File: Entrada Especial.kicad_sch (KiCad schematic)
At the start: 57 parts, among them U30 TLV9301xDBV, U31 TLV9301xDBV, U32 LM7705, U33 MCP1799T-5002H/TT

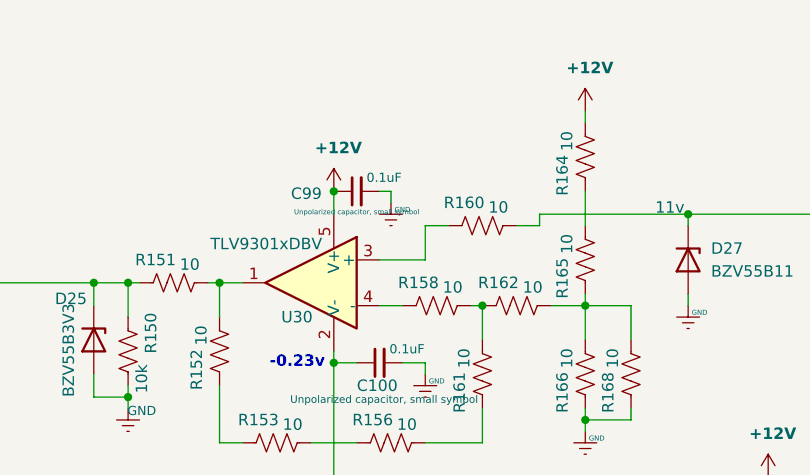
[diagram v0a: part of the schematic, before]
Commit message: 14-JUL-26
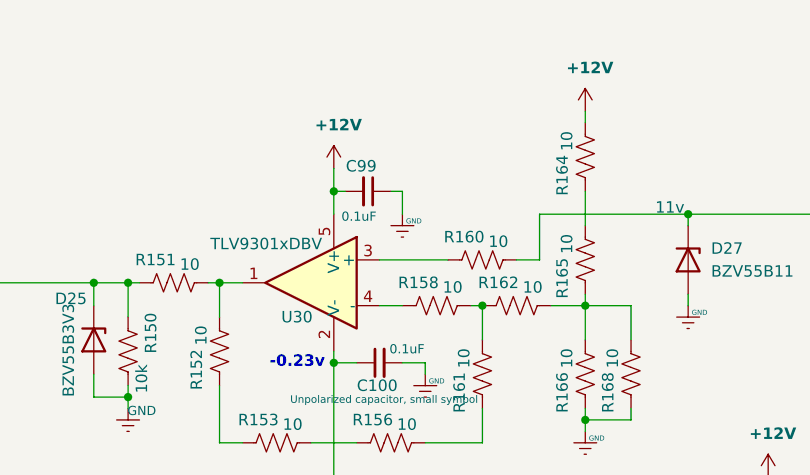
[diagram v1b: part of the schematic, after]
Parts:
- C99: now in the parts list
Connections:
- net +12V: now also C99.2; no longer C99.1
- net GND: now also C99.1; no longer C99.2
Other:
- moved on the sheet: R160
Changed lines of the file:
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@@
 	)
 	(junction
-		(at 77.47 67.31)
-		(diameter 0)
-		(color 0 0 0 0)
-	)
-	(junction
 		(at 77.47 86.36)
 		(diameter 0)
@@
 	)
 	(junction
+		(at 77.47 67.31)
+		(diameter 0)
+		(color 0 0 0 0)
+	)
+	(junction
 		(at 140.97 154.94)
 		(diameter 0)
@@
 	(wire
 		(pts
-			(xy 93.98 95.25) (xy 93.98 91.44)
+			(xy 77.47 67.31) (xy 77.47 69.85)
 		)
 		(stroke
@@
 	(wire
 		(pts
-			(xy 87.63 74.93) (xy 87.63 71.12)
+			(xy 93.98 95.25) (xy 93.98 91.44)
 		)
 		(stroke
@@
 	(wire
 		(pts
-			(xy 87.63 71.12) (xy 90.17 71.12)
-		)
-		(stroke
-			(width 0)
-			(type default)
-		)
-	)
-	(wire
-		(pts
 			(xy 243.84 102.87) (xy 251.46 102.87)
 		)
@@
 	(wire
 		(pts
-			(xy 82.55 67.31) (xy 83.82 67.31)
-		)
-		(stroke
-			(width 0)
-			(type default)
-		)
-	)
-	(wire
-		(pts
 			(xy 120.65 110.49) (xy 137.16 110.49)
 		)
@@
 	(wire
 		(pts
-			(xy 100.33 71.12) (xy 100.33 69.85)
+			(xy 100.33 74.93) (xy 100.33 69.85)
 		)
 		(stroke
@@
 	(wire
 		(pts
-			(xy 97.79 71.12) (xy 100.33 71.12)
+			(xy 97.79 74.93) (xy 100.33 74.93)
 		)
 		(stroke
@@
 	(wire
 		(pts
-			(xy 82.55 74.93) (xy 87.63 74.93)
+			(xy 82.55 74.93) (xy 90.17 74.93)
 		)
 		(stroke
@@
 	(wire
 		(pts
+			(xy 85.09 67.31) (xy 83.82 67.31)
+		)
+		(stroke
+			(width 0)
+			(type default)
+		)
+	)
+	(wire
+		(pts
 			(xy 110.49 92.71) (xy 105.41 92.71)
 		)
@@
 	(wire
 		(pts
+			(xy 78.74 67.31) (xy 77.47 67.31)
+		)
+		(stroke
+			(width 0)
+			(type default)
+		)
+	)
+	(wire
+		(pts
 			(xy 170.18 133.35) (xy 170.18 130.81)
 		)
@@
 	(wire
 		(pts
-			(xy 77.47 67.31) (xy 77.47 69.85)
+			(xy 77.47 64.77) (xy 77.47 67.31)
 		)
 		(stroke
@@
 	(wire
 		(pts
-			(xy 83.82 67.31) (xy 83.82 68.58)
+			(xy 85.09 67.31) (xy 85.09 69.85)
 		)
 		(stroke
@@
 	(symbol
 		(lib_id "power:+12V")
-		(at 77.47 67.31 0)
+		(at 77.47 64.77 0)
 		(mirror y)
 		(unit 1)
@@
 		(dnp no)
 		(property "Reference" "#PWR0364"
-			(at 77.47 71.12 0)
+			(at 77.47 68.58 0)
 			(effects
 				(font
@@
 		)
 		(property "Value" "+12V"
-			(at 77.978 62.484 0)
+			(at 77.978 59.944 0)
 			(effects
 				(font
@@
 		)
 		(property "Footprint" ""
-			(at 77.47 67.31 0)
+			(at 77.47 64.77 0)
 			(effects
 				(font
@@
 		)
 		(property "Datasheet" ""
-			(at 77.47 67.31 0)
+			(at 77.47 64.77 0)
 			(effects
 				(font
@@
 		)
 		(property "Description" "Power symbol creates a global label with name \"+12V\""
-			(at 77.47 67.31 0)
+			(at 77.47 64.77 0)
 			(effects
 				(font
@@
 	(symbol
 		(lib_id "Device:R_US")
-		(at 93.98 71.12 270)
+		(at 93.98 74.93 270)
 		(unit 1)
 		(exclude_from_sim no)
@@
 		(dnp no)
 		(property "Reference" "R160"
-			(at 91.948 68.58 90)
+			(at 91.948 72.39 90)
 			(effects
 				(font
@@
 		)
 		(property "Value" "10"
-			(at 95.758 69.088 90)
+			(at 95.758 72.898 90)
 			(effects
 				(font
@@
 		)
 		(property "Footprint" "Resistor_SMD:R_0603_1608Metric"
-			(at 93.726 72.136 90)
+			(at 93.726 75.946 90)
 			(effects
 				(font
@@
 		)
 		(property "Datasheet" "~"
-			(at 93.98 71.12 0)
+			(at 93.98 74.93 0)
 			(effects
 				(font
@@
 		)
 		(property "Description" "Resistor, US symbol"
-			(at 93.98 71.12 0)
+			(at 93.98 74.93 0)
 			(effects
 				(font
@@
 	(symbol
 		(lib_id "Device:C_Small")
+		(at 81.28 67.31 270)
+		(mirror x)
+		(unit 1)
+		(exclude_from_sim no)
+		(in_bom yes)
+		(on_board yes)
+		(dnp no)
+		(property "Reference" "C99"
+			(at 80.518 64.516 90)
+			(effects
+				(font
+					(size 1.27 1.27)
+				)
+			)
+		)
+		(property "Value" "0.1uF"
+			(at 80.264 70.104 90)
+			(effects
+				(font
+					(size 1.016 1.016)
+				)
+			)
+		)
+		(property "Footprint" "Capacitor_SMD:C_0603_1608Metric_Pad1.08x0.95mm_HandSolder"
+			(at 81.28 67.31 0)
+			(effects
+				(font
+					(size 1.27 1.27)
+				)
+				(hide yes)
+			)
+		)
+		(property "Datasheet" "~"
+			(at 81.28 67.31 0)
+			(effects
+				(font
+					(size 1.27 1.27)
+				)
+				(hide yes)
+			)
+		)
+		(property "Description" "Unpolarized capacitor, small symbol"
+			(at 81.28 67.31 0)
+			(effects
+				(font
+					(size 1.27 1.27)
+				)
+				(hide yes)
+			)
+		)
+		(pin "2"
+		)
+		(pin "1"
+		)
+		(instances
+			(project "01_IO-ASD-PLUS"
+				(path "/38a2da3c-ed29-422f-ab41-066ccf490e61/19faad97-cb14-41b6-a038-81c575645464"
+					(reference "C99")
+					(unit 1)
+				)
+			)
+		)
+	)
+	(symbol
+		(lib_id "Device:C_Small")
 		(at 204.47 135.89 0)
 		(mirror x)
@@
 	)
 	(symbol
-		(lib_id "Device:C_Small")
-		(at 80.01 67.31 90)
-		(unit 1)
-		(exclude_from_sim no)
-		(in_bom no)
-		(on_board no)
-		(dnp no)
-		(property "Reference" "C99"
-			(at 74.422 67.564 90)
-			(effects
-				(font
-					(size 1.27 1.27)
-				)
-			)
-		)
-		(property "Value" "0.1uF"
-			(at 83.058 65.786 90)
-			(effects
-				(font
-					(size 1.016 1.016)
-				)
-			)
-		)
-		(property "Footprint" "Capacitor_SMD:C_0603_1608Metric_Pad1.08x0.95mm_HandSolder"
-			(at 80.01 67.31 0)
-			(effects
-				(font
-					(size 1.27 1.27)
-				)
-				(hide yes)
-			)
-		)
-		(property "Datasheet" "~"
-			(at 80.01 67.31 0)
-			(effects
-				(font
-					(size 1.27 1.27)
-				)
-				(hide yes)
-			)
-		)
-		(property "Description" "Unpolarized capacitor, small symbol"
-			(at 80.01 69.596 90)
-			(effects
-				(font
-					(size 0.5588 0.5588)
-				)
-			)
-		)
-		(pin "2"
-		)
-		(pin "1"
-		)
-		(instances
-			(project "01_IO-ASD-PLUS"
-				(path "/38a2da3c-ed29-422f-ab41-066ccf490e61/19faad97-cb14-41b6-a038-81c575645464"
-					(reference "C99")
-					(unit 1)
-				)
-			)
-		)
-	)
-	(symbol
 		(lib_id "power:GNDREF")
 		(at 140.97 163.83 0)
@@
 	(symbol
 		(lib_id "power:GNDREF")
-		(at 83.82 68.58 0)
+		(at 85.09 69.85 0)
 		(unit 1)
 		(exclude_from_sim no)
@@
 		(dnp no)
 		(property "Reference" "#PWR0365"
-			(at 83.82 74.93 0)
+			(at 85.09 76.2 0)
 			(effects
 				(font
@@
 		)
 		(property "Value" "GND"
-			(at 85.09 69.342 0)
+			(at 86.36 70.612 0)
 			(effects
 				(font
@@
 		)
 		(property "Footprint" ""
-			(at 83.82 68.58 0)
+			(at 85.09 69.85 0)
 			(effects
 				(font
@@
 		)
 		(property "Datasheet" ""
-			(at 83.82 68.58 0)
+			(at 85.09 69.85 0)
 			(effects
 				(font
@@
 		)
 		(property "Description" "Power symbol creates a global label with name \"GNDREF\" , reference supply ground"
-			(at 83.82 68.58 0)
+			(at 85.09 69.85 0)
 			(effects
 				(font

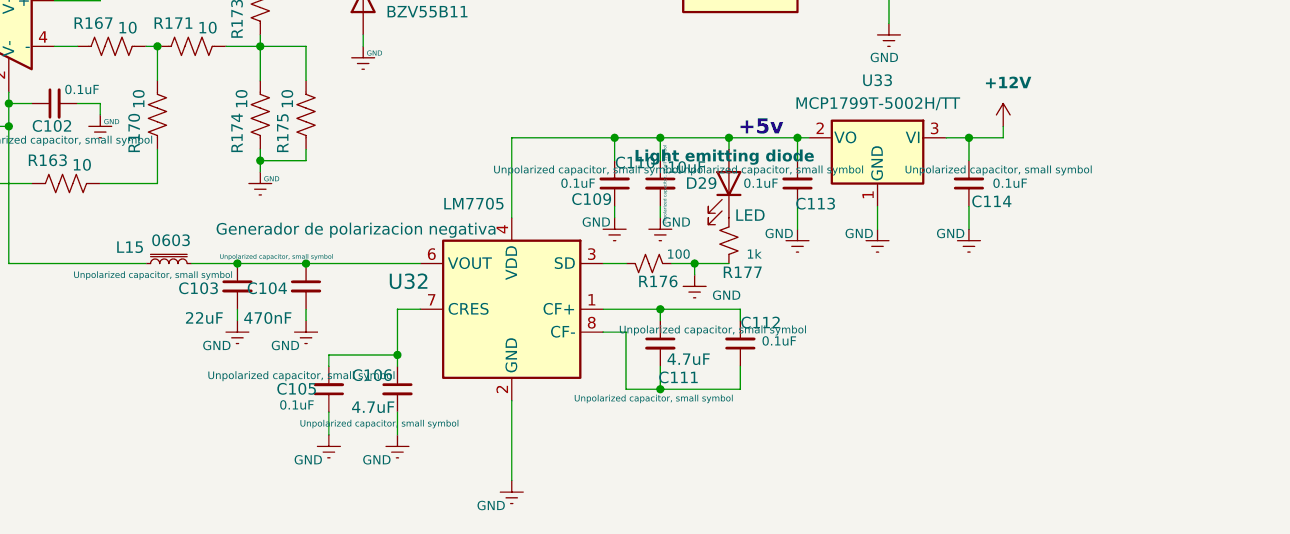
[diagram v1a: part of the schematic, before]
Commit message: 17-07-26
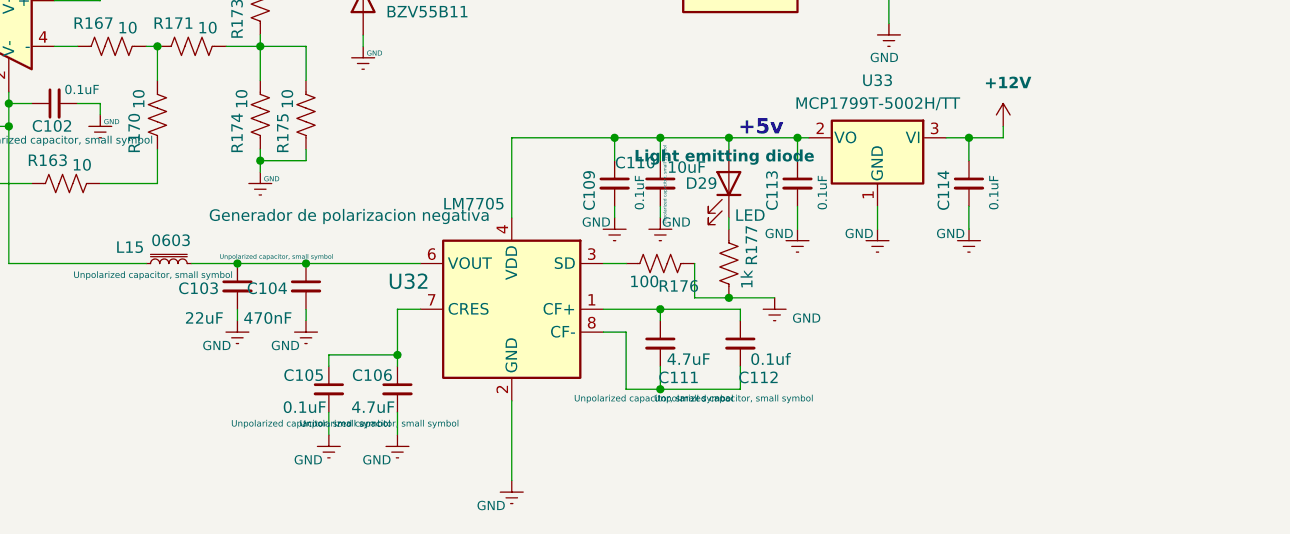
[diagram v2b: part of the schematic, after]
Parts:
- removed R176: 100, Resistor_SMD:R_0603_1608Metric_Pad0.98x0.95mm_HandSolder, symbol Device:R_Small_US
- removed R177: 1k, Resistor_SMD:R_0603_1608Metric_Pad0.98x0.95mm_HandSolder, symbol Device:R_Small_US
- added R176: 100, Resistor_SMD:R_0603_1608Metric, symbol Device:R_US
- added R177: 1k, Resistor_SMD:R_0603_1608Metric, symbol Device:R_US
- C105: footprint Capacitor_SMD:C_0603_1608Metric_Pad1.08x0.95mm_HandSolder -> Capacitor_SMD:C_0603_1608Metric; Mouser (none) -> 81-GCJ188M8EC475KE8D; Price (none) -> 0.416; now in the parts list
- C109, C113, C114: now in the parts list
- C112: value 0.1uF -> 0.1uf; footprint Capacitor_SMD:C_0603_1608Metric_Pad1.08x0.95mm_HandSolder -> Capacitor_SMD:C_0603_1608Metric; Mouser (none) -> 81-GCJ188M8EC475KE8D; Price (none) -> 0.416; now in the parts list
- D29: footprint LED_SMD:LED_0402_1005Metric -> LED_SMD:LED_0603_1608Metric_Pad1.05x0.95mm_HandSolder
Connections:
- net +12V: now also C114.1; no longer C114.2
- net GND: now also C105.2, C109.2, C113.2, C114.2, R176.2, R177.1; no longer C105.1, C109.1, C113.1, C114.1
- net at C111.1, U32.1 (CF+): now also C112.1; no longer C112.2
- net at C111.2, U32.8 (CF-): now also C112.2; no longer C112.1
- net at C110.1, D29.2 (A), U32.4 (VDD)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: now also C109.1, C113.1; no longer C109.2, C113.2
- net at C106.1, U32.7 (CRES): now also C105.1; no longer C105.2
- net at D29.1 (K): now also R177.2
- net at U32.3 (SD): now also R176.1
